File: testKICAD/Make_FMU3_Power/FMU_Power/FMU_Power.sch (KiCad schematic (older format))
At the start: 10 parts

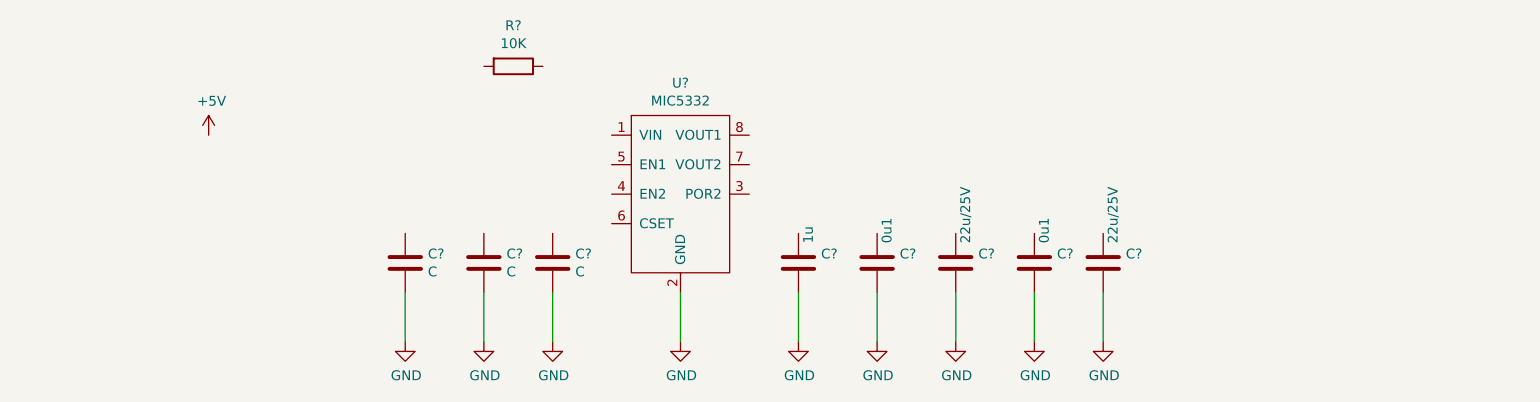
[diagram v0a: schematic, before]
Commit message: FMU3 Power make
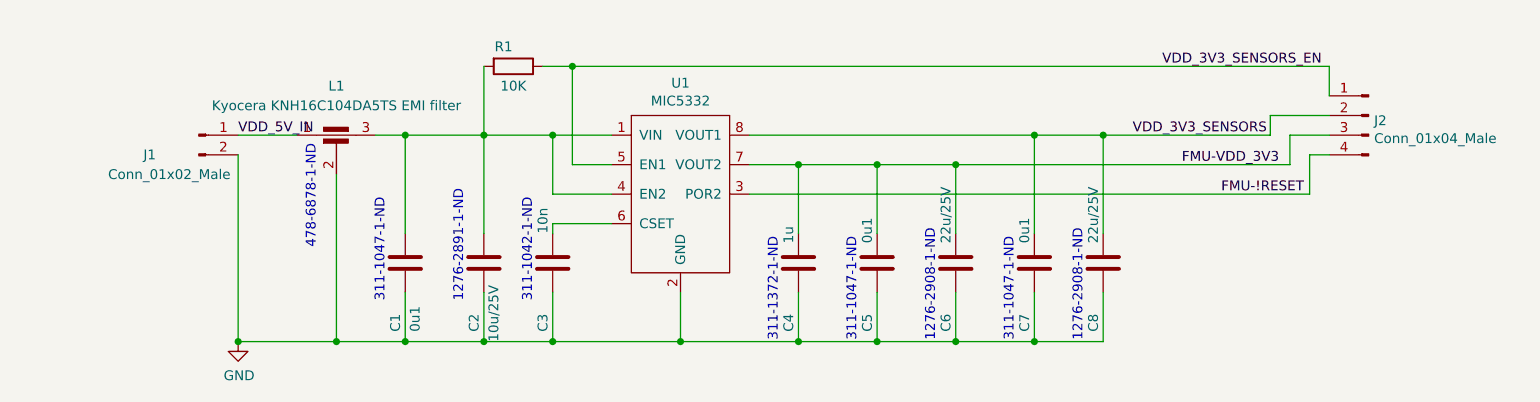
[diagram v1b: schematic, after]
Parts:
- added J1: Conn_01x02_Male, Connector_PinHeader_2.54mm:PinHeader_1x02_P2.54mm_Vertical_SMD_Pin1Left, symbol Connector:Conn_01x02_Male
- added J2: Conn_01x04_Male, Connector_PinHeader_2.54mm:PinHeader_1x04_P2.54mm_Vertical_SMD_Pin1Left, symbol Connector:Conn_01x04_Male
- added L1: Kyocera KNH16C104DA5TS EMI filter, wooslib:KNH16C104DA5TS_EMI_filter, symbol Device:EMI_Filter_C
- C1: renamed from C?; value C -> 0u1; footprint (none) -> wooslib:CC0402ZRY5V7BB104_1.0x0.5mm
- C2: renamed from C?; value C -> 10u/25V; footprint (none) -> wooslib:CL21A106KAYNNNE_2.0x1.25mm
- C3: renamed from C?; value C -> 10n; footprint (none) -> wooslib:CC0402KRX7R7BB103_1.0x0.5mm
- C4: renamed from C?; footprint (none) -> wooslib:CC0603ZRY5V7BB105_1.6x0.8
- C5, C7: renamed from C?; footprint (none) -> wooslib:CC0402ZRY5V7BB104_1.0x0.5mm
- C6, C8: renamed from C?; footprint (none) -> wooslib:CL21A226MAQNNNE_2.0x1.25mm
- R1: renamed from R?; footprint (none) -> wooslib:RC0402FR-0710KL_1.0x0.5mm
- U1: renamed from U?; footprint (none) -> wooslib:MIC5332
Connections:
- net GND: now also J1.2 (Pin_2), L1.2
- net at U1.1 (VIN): now also C1.1, C2.1, R1.2, U1.4 (EN2), L1.3
- net FMU-!RESET: now reaches U1.3 (POR2)
- net FMU-!RESET: now also J2.4 (Pin_4)
- net VDD_3V3_SENSORS_EN: now reaches U1.5 (EN1)
- net VDD_3V3_SENSORS_EN: now also R1.1, J2.1 (Pin_1)
- net at U1.6 (CSET): now also C3.1
- net FMU-VDD_3V3: now reaches U1.7 (VOUT2)
- net FMU-VDD_3V3: now also C4.1, C5.1, C6.1, J2.3 (Pin_3)
- net VDD_3V3_SENSORS: now reaches U1.8 (VOUT1)
- net VDD_3V3_SENSORS: now also C7.1, C8.1, J2.2 (Pin_2)
- new net VDD_5V_IN: J1.1 (Pin_1), L1.1
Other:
- note added: "1276-2891-1-ND"
- note added: "1276-2908-1-ND"
- note added: "311-1042-1-ND"
- note added: "311-1047-1-ND"
- note added: "311-1372-1-ND"
- note added: "478-6878-1-ND"

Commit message: adding files
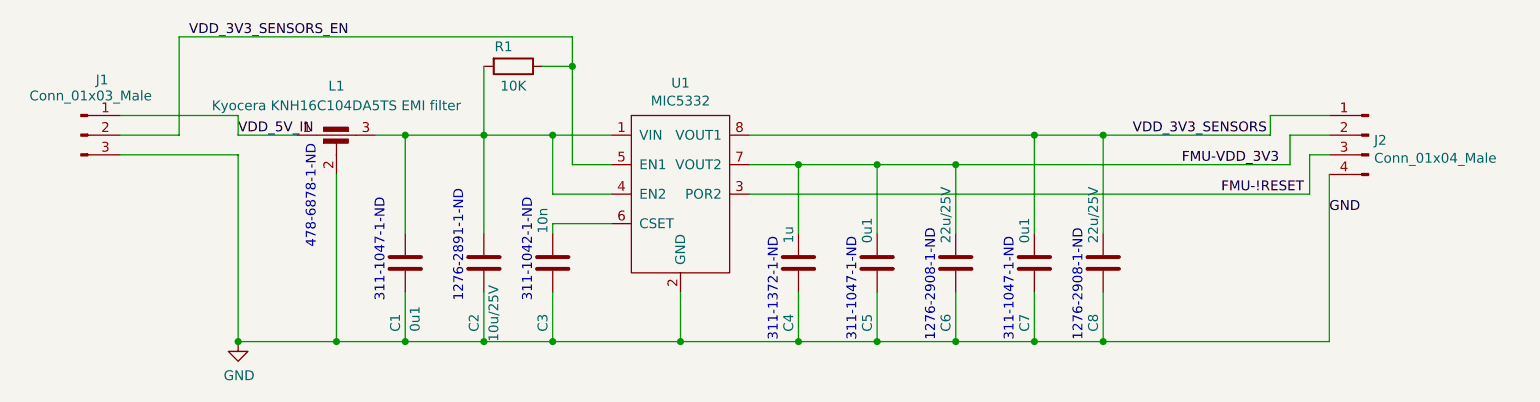
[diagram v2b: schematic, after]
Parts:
- removed J1: Conn_01x02_Male, Connector_PinHeader_2.54mm:PinHeader_1x02_P2.54mm_Vertical_SMD_Pin1Left, symbol Connector:Conn_01x02_Male
- added J1: Conn_01x03_Male, wooslib:MIC5332_INPUT_Connectpr_1x3, symbol Connector:Conn_01x03_Male
- J2: footprint Connector_PinHeader_2.54mm:PinHeader_1x04_P2.54mm_Vertical_SMD_Pin1Left -> wooslib:MIC5332_OUTPUT_Connector
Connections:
- net FMU-!RESET: now also J2.3 (Pin_3); no longer J2.4 (Pin_4)
- net FMU-VDD_3V3: now also J2.2 (Pin_2); no longer J2.3 (Pin_3)
- net GND: now also J2.4 (Pin_4), J1.3 (Pin_3)
- net VDD_3V3_SENSORS: now also J2.1 (Pin_1); no longer J2.2 (Pin_2)
- net VDD_3V3_SENSORS_EN: now also J1.2 (Pin_2); no longer J2.1 (Pin_1)
- net VDD_5V_IN: now also J1.1 (Pin_1)
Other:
- moved on the sheet: J2
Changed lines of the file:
@@
 Wire Wire Line
 	3900 3950 3900 3450
-Text Label 7750 3100 0    50   ~ 0
+Text Label 2800 2950 0    50   ~ 0
 VDD_3V3_SENSORS_EN
 Text Label 7600 3450 0    50   ~ 0
@@
 L Connector:Conn_01x04_Male J2
 U 1 1 5EC5E87A
-P 8800 3350
-F 0 "J2" H 8772 3324 50  0000 R CNN
-F 1 "Conn_01x04_Male" H 8772 3233 50  0000 R CNN
-F 2 "Connector_PinHeader_2.54mm:PinHeader_1x04_P2.54mm_Vertical_SMD_Pin1Left" H 8800 3350 50  0001 C CNN
-F 3 "~" H 8800 3350 50  0001 C CNN
-	1    8800 3350
+P 8800 3450
+F 0 "J2" H 8772 3424 50  0000 R CNN
+F 1 "Conn_01x04_Male" H 8772 3333 50  0000 R CNN
+F 2 "wooslib:MIC5332_OUTPUT_Connector" H 8800 3450 50  0001 C CNN
+F 3 "~" H 8800 3450 50  0001 C CNN
+	1    8800 3450
 	-1   0    0    -1
 $EndComp
-Wire Wire Line
-	8600 3100 8600 3250
-Wire Wire Line
-	4750 3100 8600 3100
 Wire Wire Line
 	8300 3450 8300 3350
@@
 Wire Wire Line
 	5650 3750 8500 3750
-$Comp
-L Connector:Conn_01x02_Male J1
-U 1 1 5EC3E655
-P 2850 3450
-F 0 "J1" H 2600 3350 50  0000 C CNN
-F 1 "Conn_01x02_Male" H 2700 3250 50  0000 C CNN
-F 2 "Connector_PinHeader_2.54mm:PinHeader_1x02_P2.54mm_Vertical_SMD_Pin1Left" H 2850 3450 50  0001 C CNN
-F 3 "~" H 2850 3450 50  0001 C CNN
-	1    2850 3450
-	1    0    0    -1
-$EndComp
 Wire Wire Line
 	7450 4500 7100 4500
@@
 	7100 4500 6700 4500
 Connection ~ 3050 4500
+Wire Wire Line
+	7450 4500 8600 4500
+Wire Wire Line
+	8600 4500 8600 3650
+Connection ~ 7450 4500
+Text Label 8600 3850 0    50   ~ 0
+GND
+$Comp
+L Connector:Conn_01x03_Male J1
+U 1 1 5EC61786
+P 2250 3450
+F 0 "J1" H 2358 3731 50  0000 C CNN
+F 1 "Conn_01x03_Male" H 2300 3650 50  0000 C CNN
+F 2 "wooslib:MIC5332_INPUT_Connectpr_1x3" H 2250 3450 50  0001 C CNN
+F 3 "~" H 2250 3450 50  0001 C CNN
+	1    2250 3450
+	1    0    0    -1
+$EndComp
+Wire Wire Line
+	4750 3100 4750 2950
+Wire Wire Line
+	4750 2950 2750 2950
+Wire Wire Line
+	2750 2950 2750 3450
+Wire Wire Line
+	2750 3450 2450 3450
+Wire Wire Line
+	3050 3550 2450 3550
+Wire Wire Line
+	3050 3450 3050 3350
+Wire Wire Line
+	3050 3350 2450 3350
 $EndSCHEMATC
